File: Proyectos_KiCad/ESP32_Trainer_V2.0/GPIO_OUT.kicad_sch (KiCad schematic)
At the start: 31 parts, among them J10 LOAD, J2 RELE, J9 LOAD, K1 SANYOU_SRD_Form_C, Q1 2N3904, Q2 2N3904, Q3 2N3904, Q4 IRFZ44N, Q5 2N3904, Q6 IRFZ44N, U4 PC817

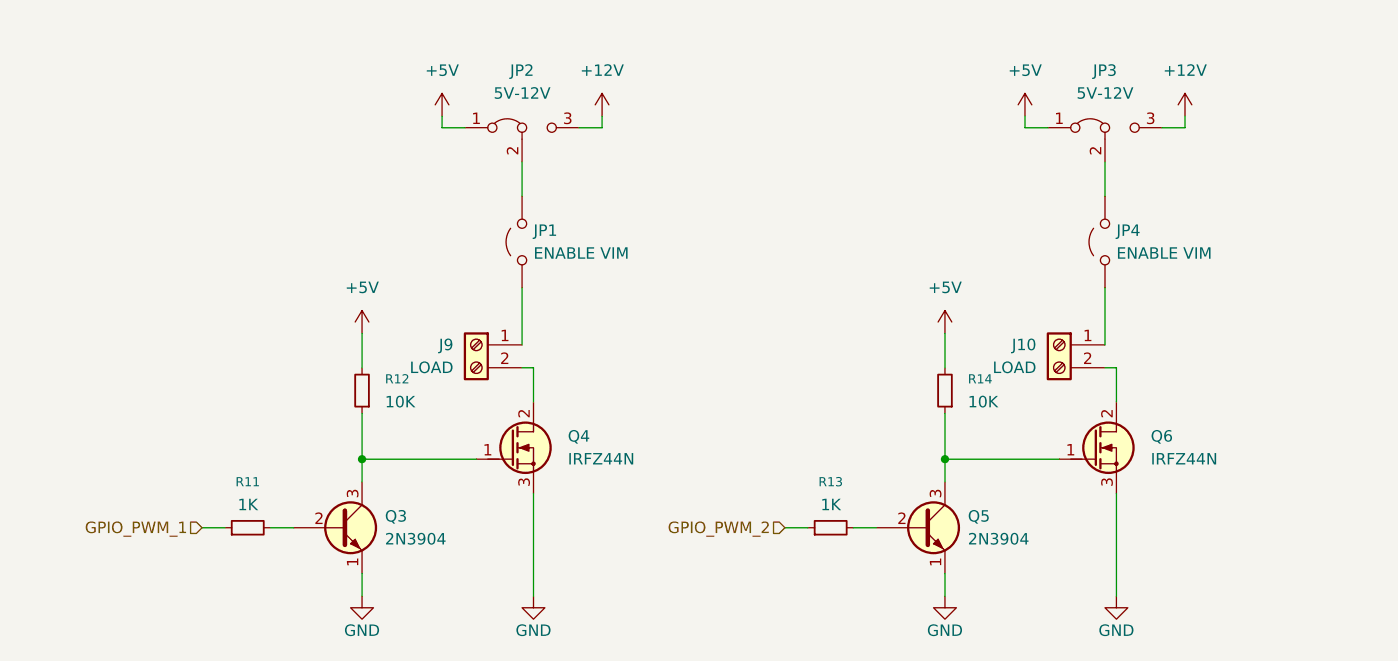
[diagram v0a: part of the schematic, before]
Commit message: Placa Entrenadora V2
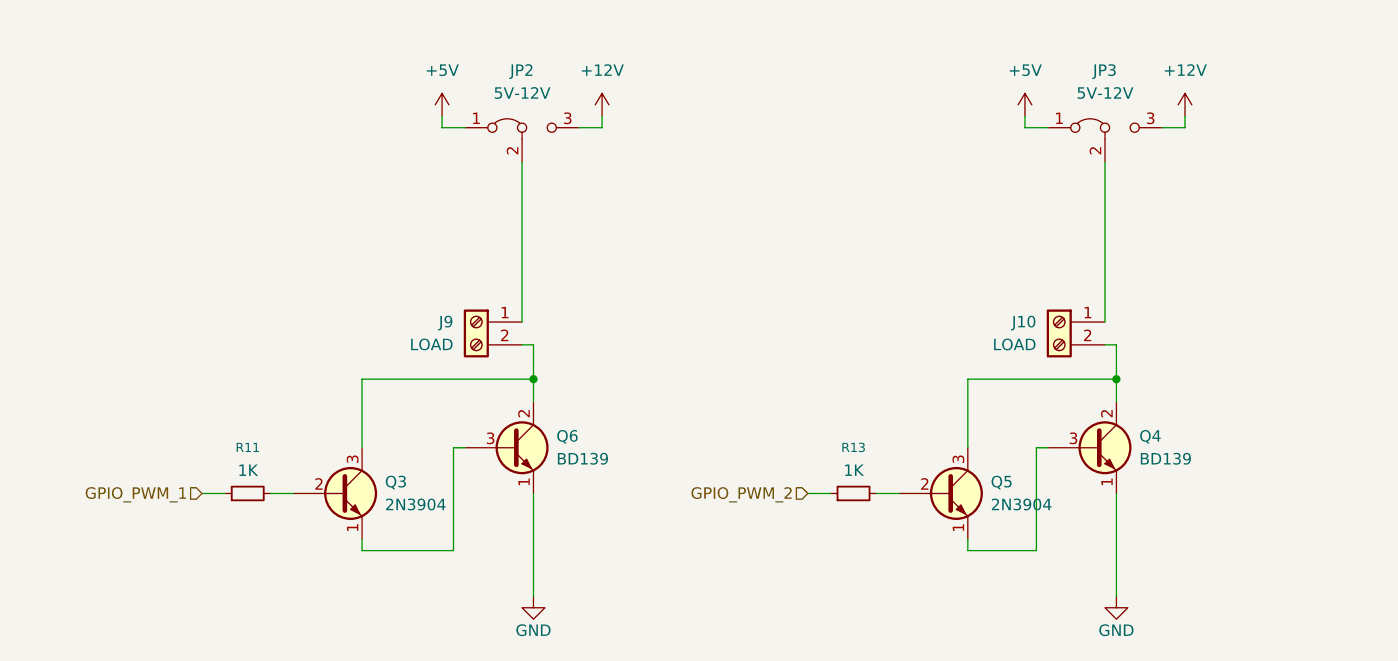
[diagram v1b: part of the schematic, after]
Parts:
- removed JP1, JP4: ENABLE VIM, PCM_SL_Connectors:PinHeader_1x03_P2.54mm_Vertical, symbol Jumper:Jumper_2_Open
- removed Q4, Q6: IRFZ44N, PCM_Package_TO_SOT_THT_AKL:TO-220-3_Vertical_GDS, symbol PCM_Transistor_MOSFET_AKL:IRFZ44N
- removed R12, R14: 10K, PCM_Resistor_SMD_AKL:R_0805_2012Metric_Pad1.15x1.40mm, symbol Device:R_Small
- added Q4, Q6: BD139, PCM_Package_TO_SOT_THT_AKL:TO-126-3_Vertical_ECB, symbol PCM_Transistor_BJT_AKL:BD139
- D7: footprint PCM_Diode_THT_AKL:D_DO-41_SOD81_P7.62mm_Horizontal -> PCM_Diode_SMD_AKL:D_SMA_BigPads
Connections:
- net GND: now also Q4.1 (E), Q6.1 (E); no longer Q3.1 (E), Q5.1 (E)
- net at J9.1 (Pin_1): now also JP2.2 (C)
- net at J9.2 (Pin_2): now also Q3.3 (C), Q6.2 (C)
- net at Q5.3 (C): now also J10.2 (Pin_2), Q4.2 (C)
- net at JP3.2 (C): now also J10.1 (Pin_1)
- new net: Q4.3 (B), Q5.1 (E)
- new net: Q3.1 (E), Q6.3 (B)
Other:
- moved on the sheet: J10, J9, Q3, Q5, R11, R13
